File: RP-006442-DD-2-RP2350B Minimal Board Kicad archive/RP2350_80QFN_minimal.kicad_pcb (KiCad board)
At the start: 2 copper layers, 99.4 x 99.4 mm, 166 parts, among them J1 USB_C_Receptacle_USB2.0_16P, J2 Conn_02x14_Odd_Even, J3 Conn_02x09_Odd_Even, J4 Conn_01x03, J5 USB_C_Receptacle_USB2.0_16P, J6 Conn_01x05, SW1 SW_Push, SW10 SW_DIP_x08, SW2 SW_Push, SW3 SW_Push, SW4 SW_Push, SW5 SW_Push, SW6 SW_Push, SW7 SW_Push, SW8 SW_Push, SW9 SW_SPDT, U1 RP2350_80QFN, U10 74HC595, U11 74HC595, U12 74HC595, U13 MMA8451QR1, U14 GS3011CR-G, U15 GS3011CR-G, U16 GS3011CR-G, U17 GS3011CR-G, U2 NCP1117-3.3_SOT223, U3 W25Q128JVS, U4 DNF, U5 W25Q128JVS, U6 NCP1117-3.3_SOT223, U7 RP2350_60QFN, U8 HT16K33A-24SSOP, Y1 ABM8-272-T3, Y2 ABM8-272-T3

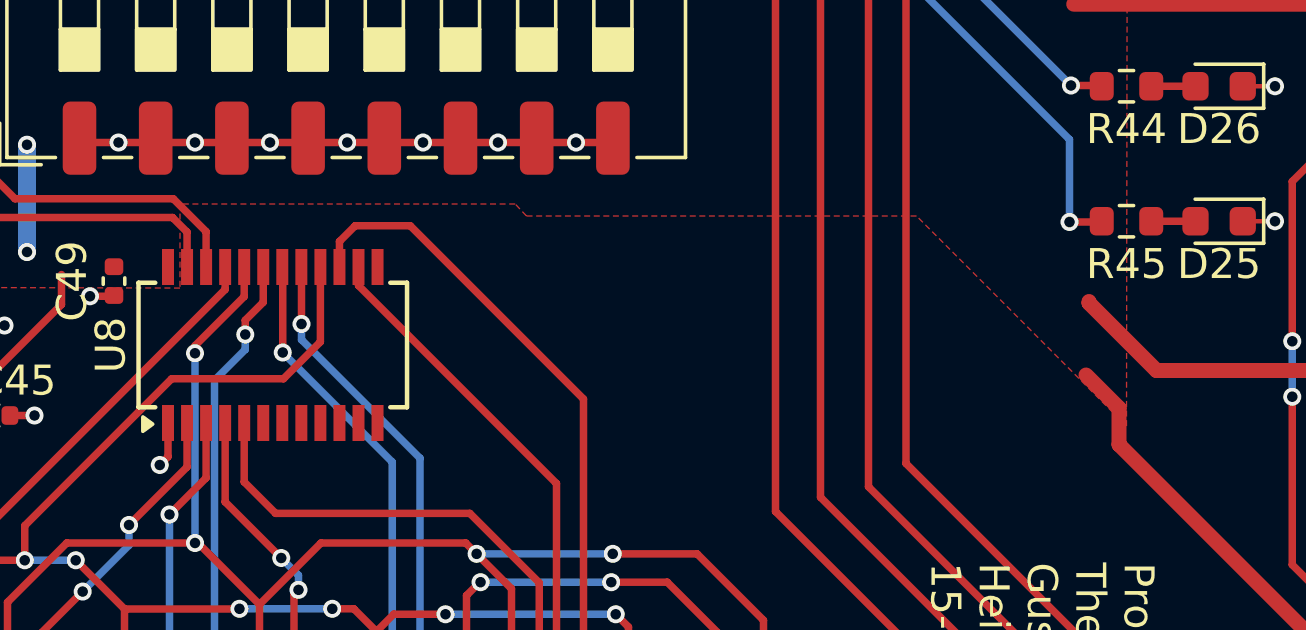
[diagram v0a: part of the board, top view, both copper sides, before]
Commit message: Update
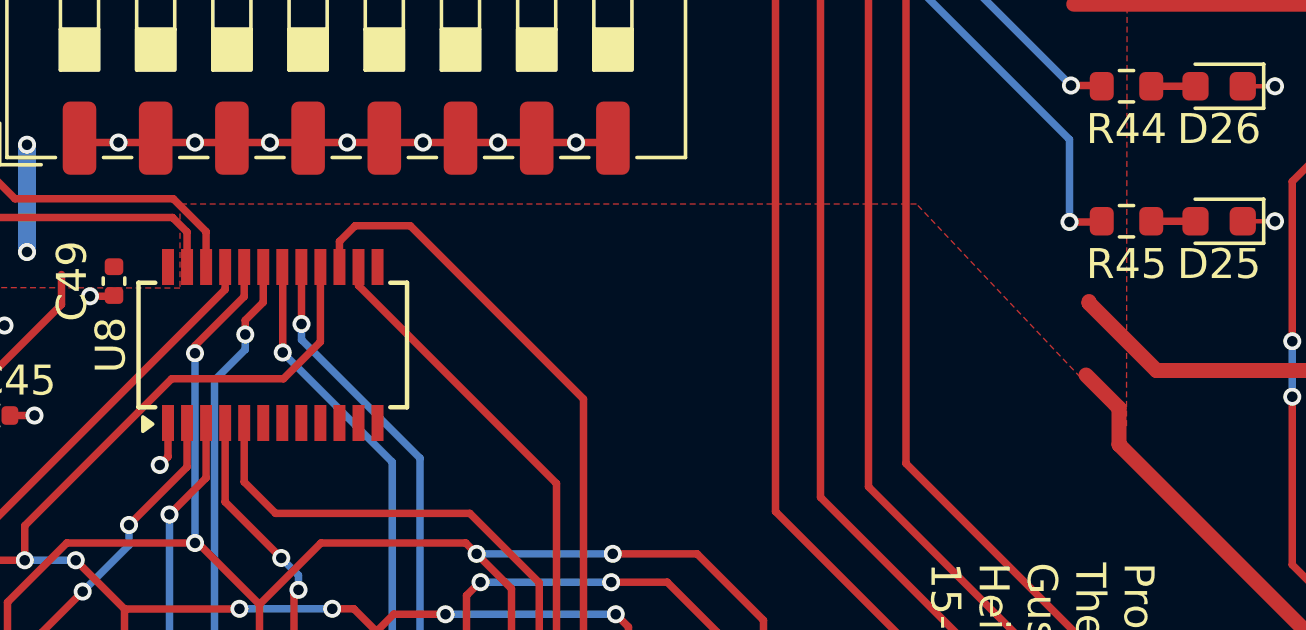
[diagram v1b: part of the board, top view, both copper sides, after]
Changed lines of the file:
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@@
 		(polygon
 			(pts
-				(xy 60.975 44.35) (xy 113.3 44.475) (xy 113.199715 116.35) (xy 106.20145 109.35) (xy 93.2 109.35)
-				(xy 92.824238 108.95) (xy 81.65 108.95) (xy 81.65 111.751877) (xy 60.675 111.7)
+				(xy 60.975 44.35) (xy 113.3 44.475) (xy 113.199715 116.35) (xy 106.2 108.95) (xy 81.65 108.95) (xy 81.65 111.751877)
+				(xy 60.675 111.7)
 			)
 		)
